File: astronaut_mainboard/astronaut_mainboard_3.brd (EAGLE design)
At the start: 69.5 x 52.1 mm, 23 parts, among them IC1 ADUM1250, IC2 741G3157DBVR, IC3 741G3157DBVR, J10 HF Comm, J6 Ext 5V, J7 UI, J8 Arduino (DWM), J9 GNSS, Q1 BSS138, Q3 BSS138

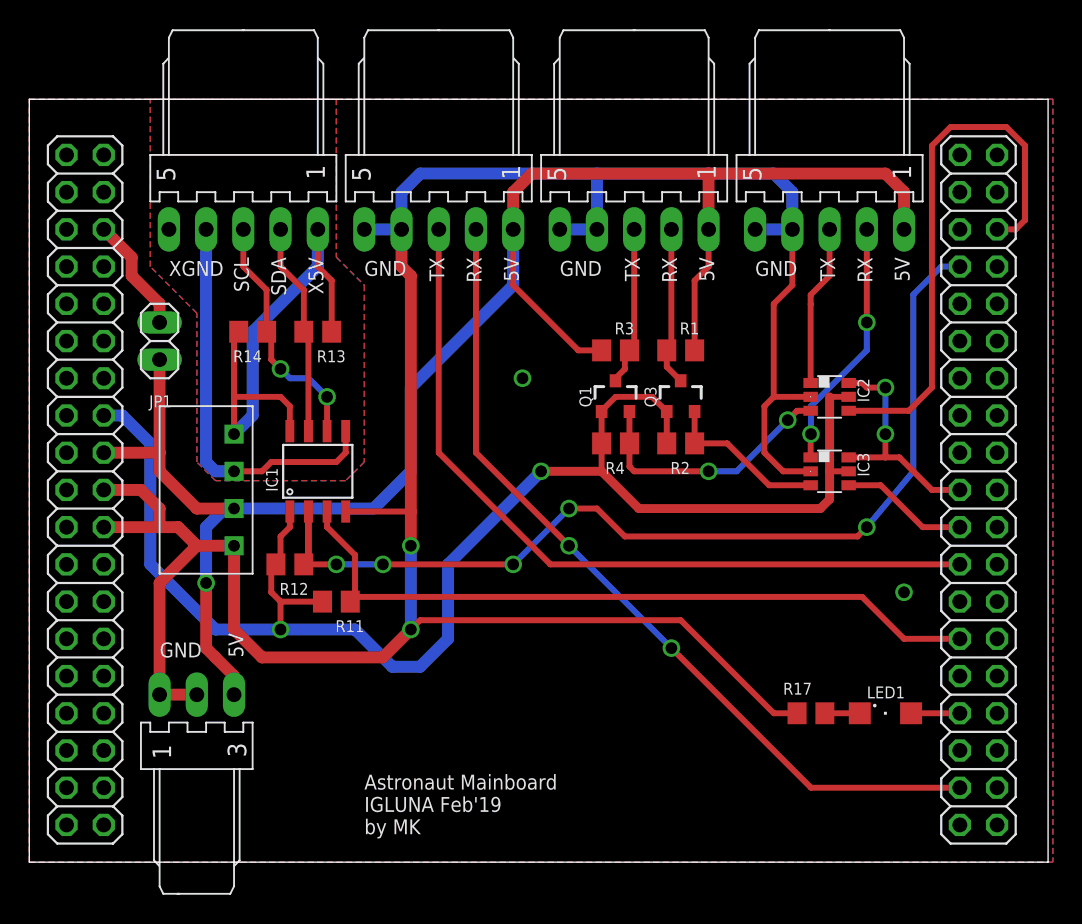
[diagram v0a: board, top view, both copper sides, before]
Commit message: final, after another review
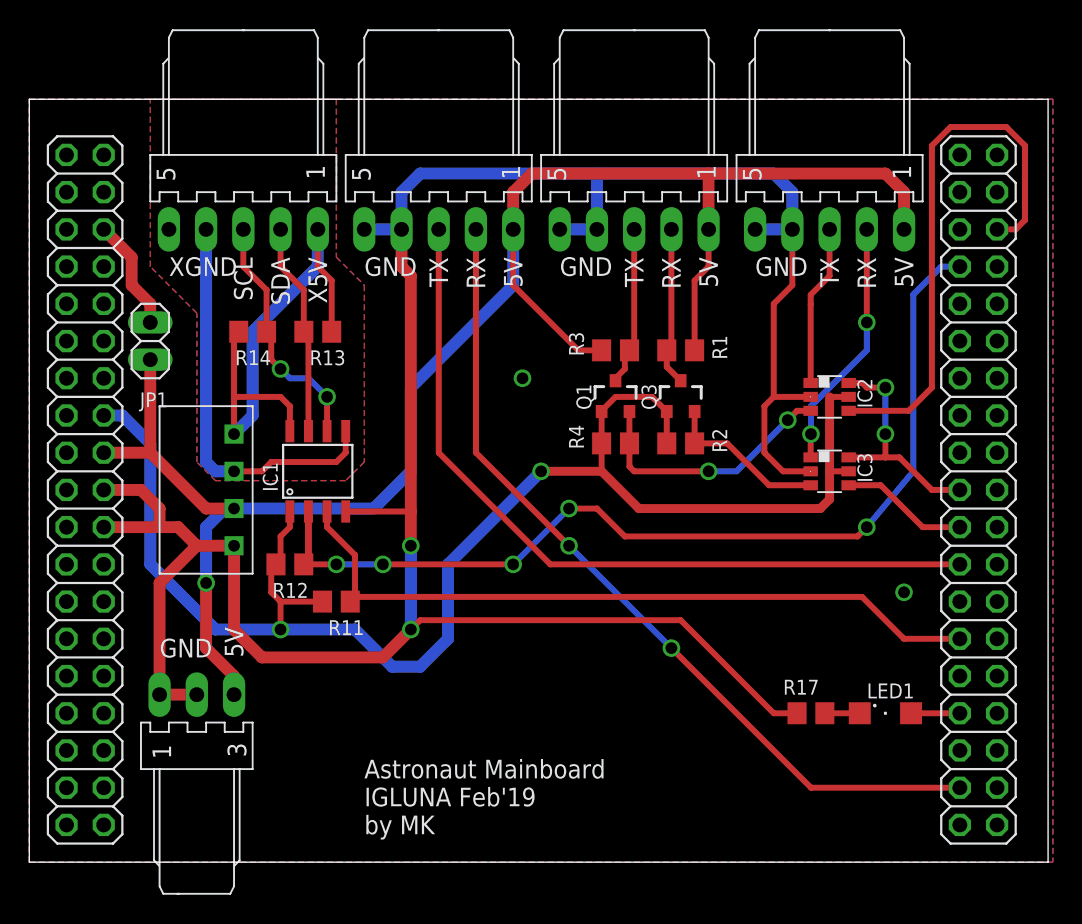
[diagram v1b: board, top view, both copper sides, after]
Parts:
- moved JP1 0.63 mm to (9.53, 35.6)
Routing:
- net +5V: track 121.7 -> 120.9 mm
